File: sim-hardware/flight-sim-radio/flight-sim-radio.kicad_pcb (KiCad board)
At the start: 2 copper layers, 170 x 45 mm, 26 parts, among them J1 Conn_01x03, J2 Conn_01x09, J3 Conn_01x04, SW1 RS-08 300±150GF, SW2 RotaryEncoder_Switch, SW3 RotaryEncoder_Switch, U1 74LS148, U2 TM1637, U3 TM1637

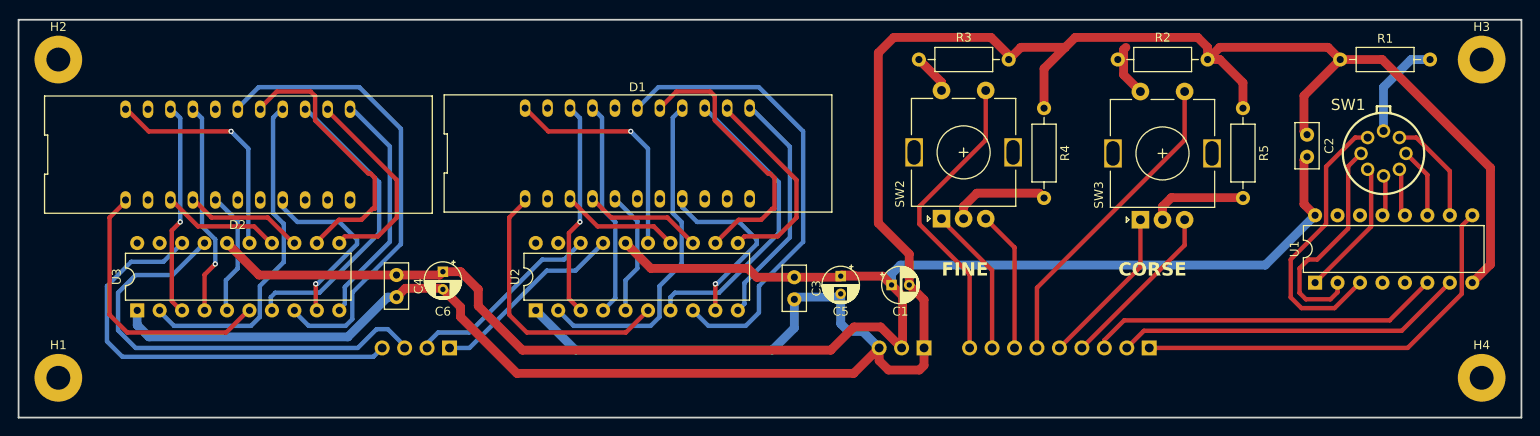
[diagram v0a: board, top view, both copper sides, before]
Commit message: PCB checked
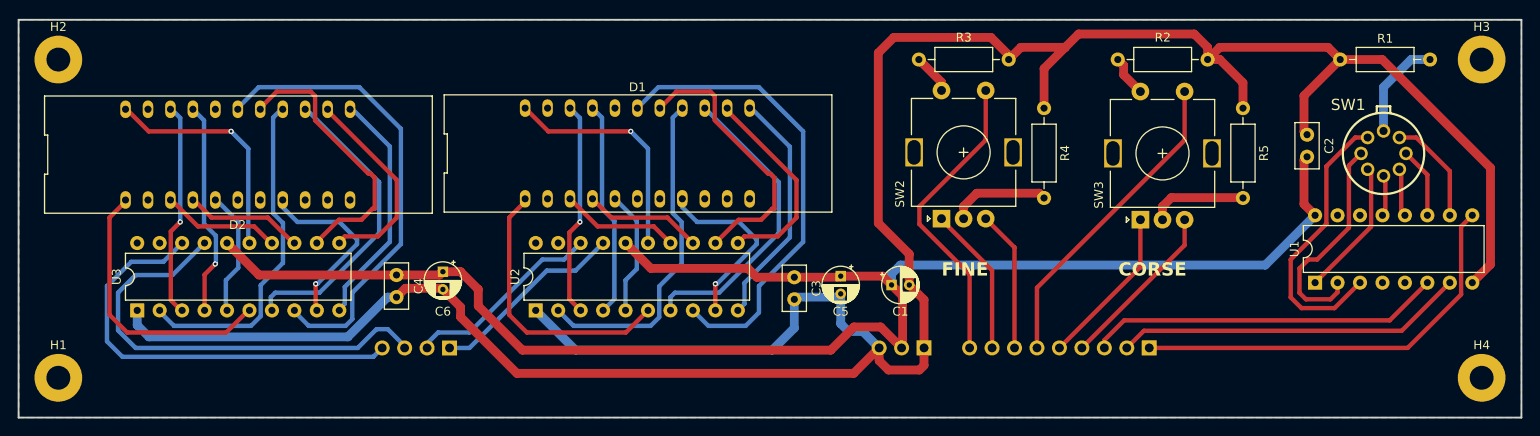
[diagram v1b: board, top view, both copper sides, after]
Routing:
- net VDD: track 185.4 -> 183.8 mm
- net Net-(R2-Pad2): track 5.89 -> 4.68 mm
- added copper zone on B.Cu, net GND
- added copper zone on F.Cu, net GND
